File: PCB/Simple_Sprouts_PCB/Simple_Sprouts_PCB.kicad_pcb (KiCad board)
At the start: 4 copper layers, 56 x 66.5 mm, 29 parts, among them J1 Simple Sprouts PCB, Q1 IRLB8721PbF, Q2 IRLB8721PbF, Q3 IRLB8721PbF, Q4 IRLB8721PbF, Q5 IRLB8721PbF, Q6 IRLB8721PbF

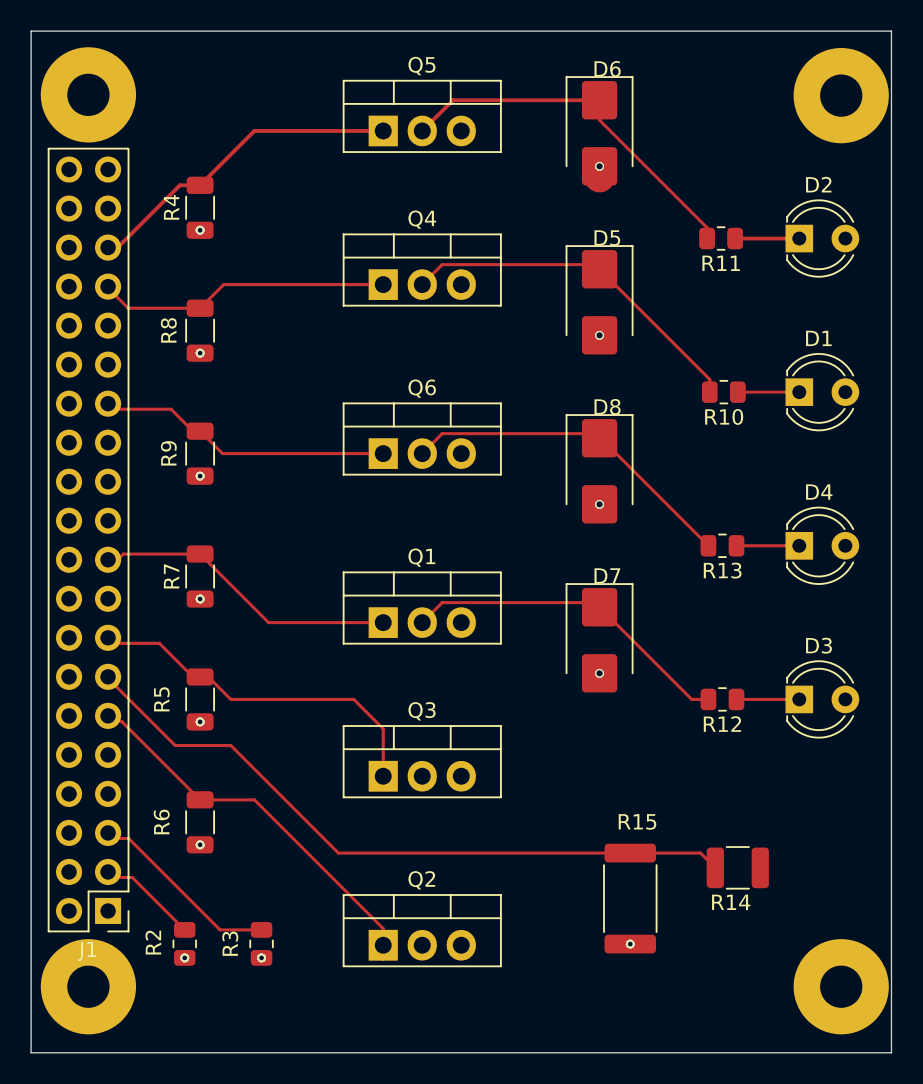
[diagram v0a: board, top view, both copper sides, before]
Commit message: Add files via upload
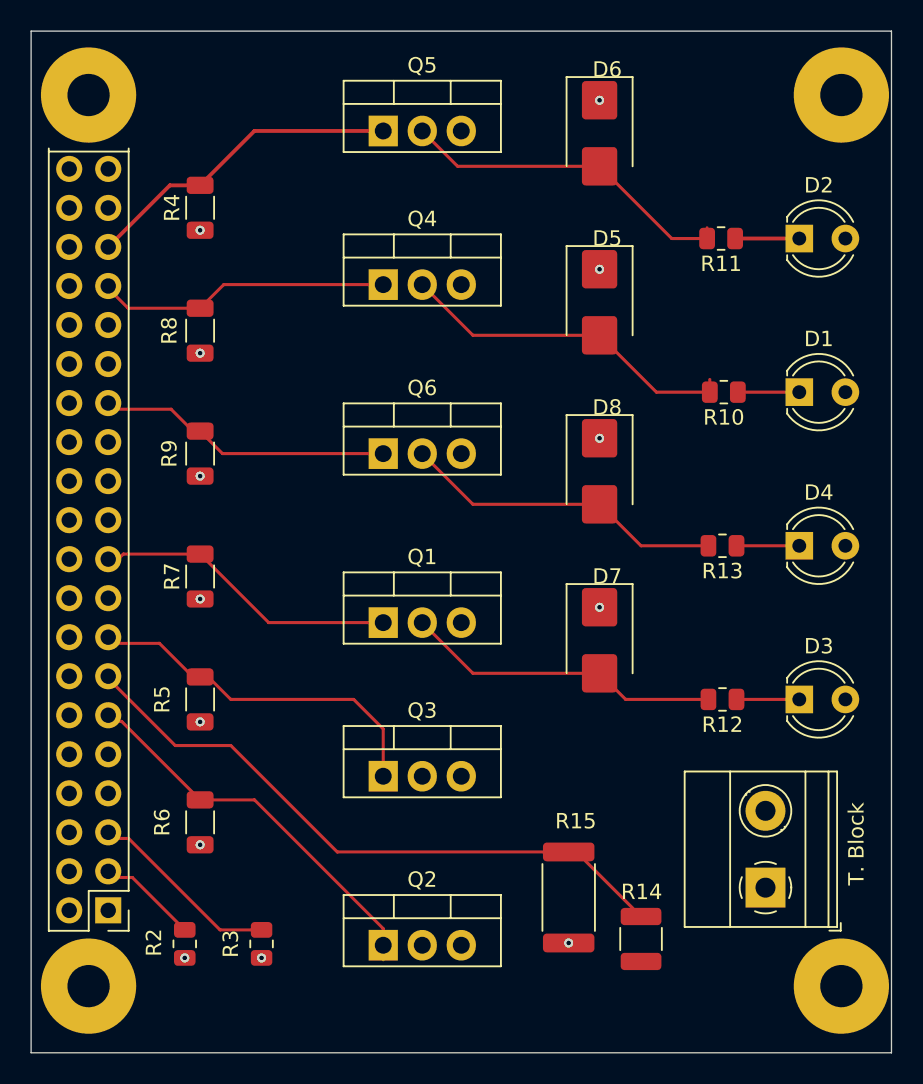
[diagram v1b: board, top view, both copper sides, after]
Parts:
- removed J1: Simple Sprouts PCB, RASPBERRY_PI_4B_4GB:Pin_Replacement
- added REF**: Pin_Replacement, RASPBERRY_PI_4B_4GB:Pin_Replacement, F.Cu at (120.9, 72.3)
- added T. Block: TerminalBlock_Phoenix_MKDS-1,5-2_1x02_P5.00mm_Horizontal, TerminalBlock_Phoenix:TerminalBlock_Phoenix_MKDS-1,5-2_1x02_P5.00mm_Horizontal, F.Cu at (167.1, 116.5)
- R4, R5, R6, R7, R8, R9: value 220Ω -> 10kΩ
- moved R14 7.82 mm to (159.0, 119.9), turned to -90 degrees
- moved R15 4.01 mm to (154.3, 117.2)
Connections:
- D5 pad 1: Net-(D5-K) -> +12V
- D5 pad 2: +12V -> Net-(D5-A)
- D6 pad 1: Net-(D6-K) -> +12V
- D6 pad 2: +12V -> Net-(D6-A)
- D7 pad 1: Net-(D7-K) -> +12V
- D7 pad 2: +12V -> Net-(D7-A)
- D8 pad 1: Net-(D8-K) -> +12V
- D8 pad 2: +12V -> Net-(D8-A)
- Q1 pad 2: Net-(D7-K) -> Net-(D7-A)
- Q4 pad 2: Net-(D5-K) -> Net-(D5-A)
- Q5 pad 2: Net-(D6-K) -> Net-(D6-A)
- Q6 pad 2: Net-(D8-K) -> Net-(D8-A)
- R10 pad 2: Net-(D5-K) -> Net-(D5-A)
- R11 pad 2: Net-(D6-K) -> Net-(D6-A)
- R12 pad 2: Net-(D7-K) -> Net-(D7-A)
- R13 pad 2: Net-(D8-K) -> Net-(D8-A)
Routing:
- net +12V: track 98.4 -> 136.2 mm
- net Net-(D6-K): track 24.3 -> 0.00 mm
- net Net-(D5-K): track 23.2 -> 0.00 mm
- net Net-(D5-A): track 0.00 -> 22.4 mm
- net Net-(D8-K): track 22.2 -> 0.00 mm
- net Net-(D6-A): track 0.00 -> 22.1 mm
- net Net-(D7-K): track 21.8 -> 0.00 mm
- net Net-(D8-A): track 0.00 -> 21.1 mm
- net Net-(D7-A): track 0.00 -> 20.7 mm
- net Net-(J1-GPIO27/SDIO_DAT3): track 44.8 -> 40.8 mm
- net GND: track 150.4 -> 146.9 mm
